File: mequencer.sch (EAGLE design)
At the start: 62 parts, among them IC1 NE555D, IC10 LF353D, IC11 NE555D, IC12 NE555D, IC2 4163D, IC3 74HC85D, IC4 4051D, IC5 4051D, IC6 74HCT04D, IC7 4051D, IC8 4051D, IC9 LF353D, U1 74LVC1G08SE-7

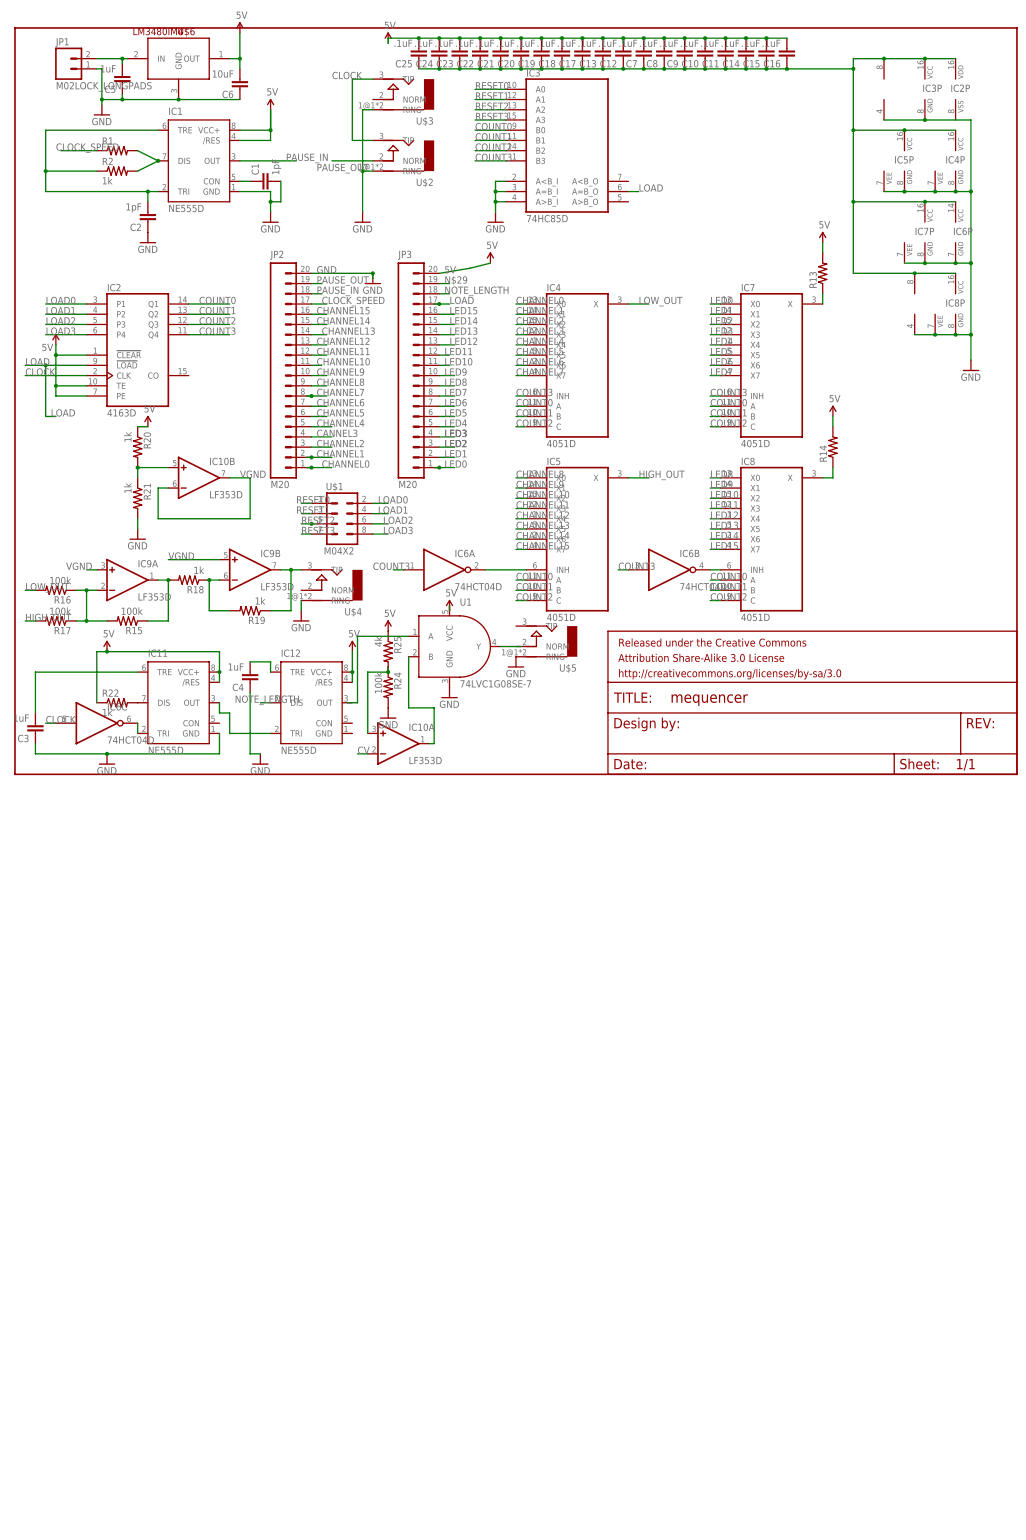
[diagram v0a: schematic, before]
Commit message: mini boards
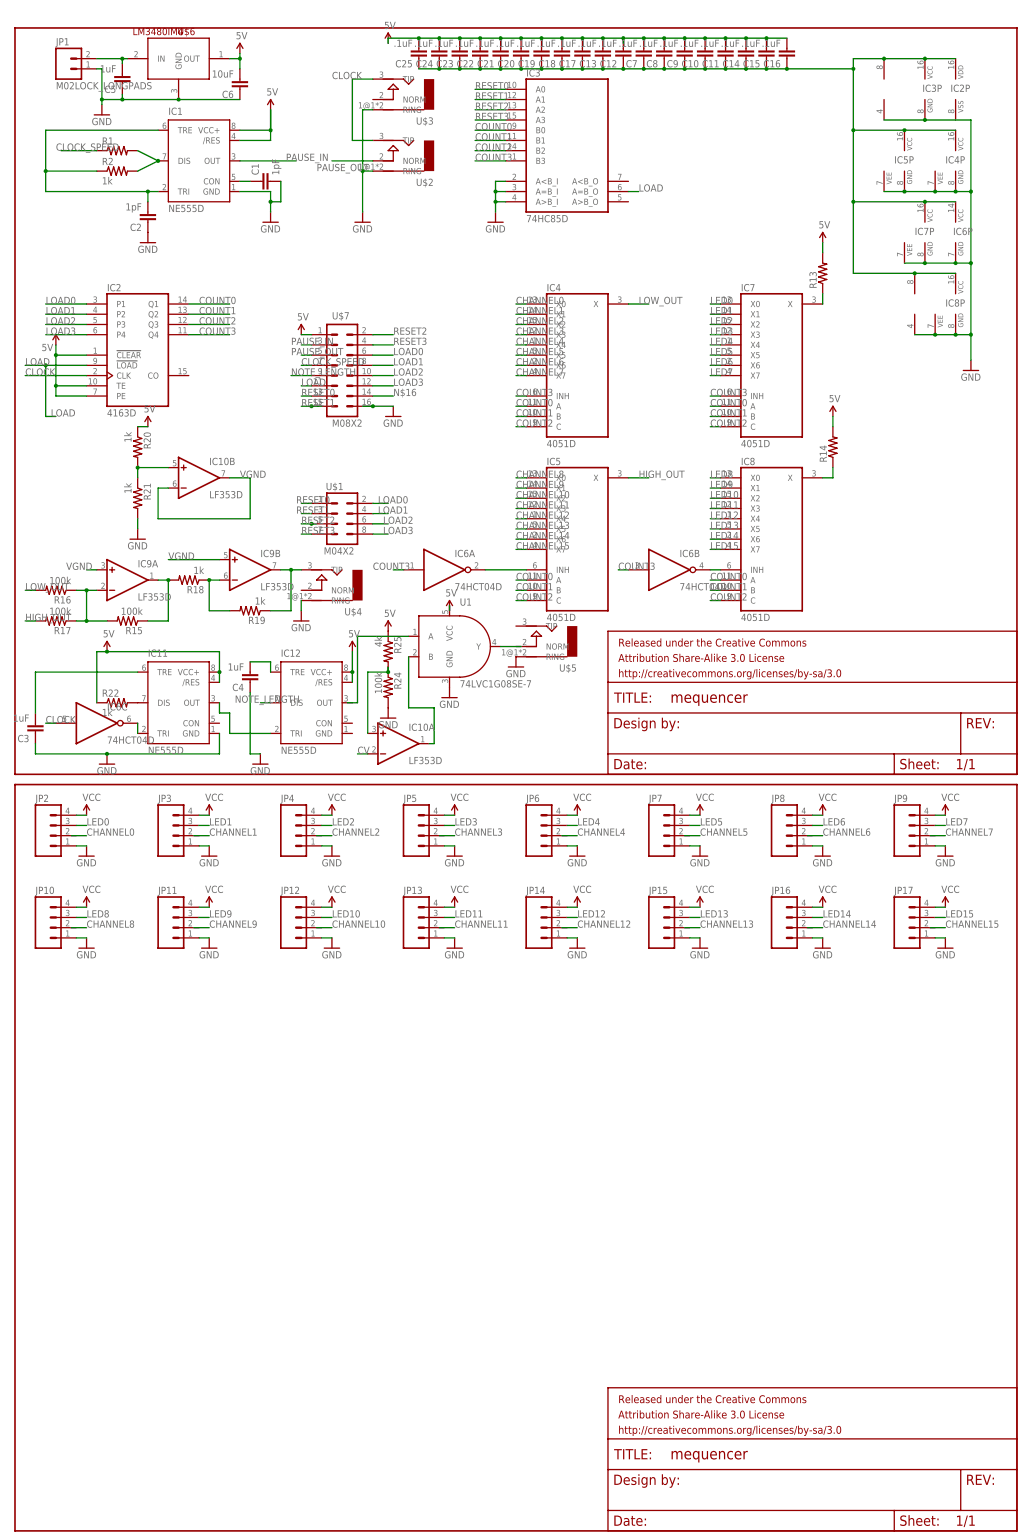
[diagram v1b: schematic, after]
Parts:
- added FRAME2: FRAME-LETTER, SparkFun-Aesthetics:FRAME-LETTER
- added JP10, JP11, JP12, JP13, JP14, JP15, JP16, JP17, JP4, JP5, JP6, JP7, JP8, JP9: (no value), SparkFun-Connectors:M04JST-PTH
- added U$7: M08X2, SparkFun-Connectors:M08X2
- JP2, JP3: value M20 -> (none); device SparkFun-Connectors:M20 -> SparkFun-Connectors:M04JST-PTH
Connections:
- removed net CANNEL3: JP2.4
- removed net N$29: JP3.19
- new net VCC: JP10.4, JP11.4, JP12.4, JP13.4, JP14.4, JP15.4, JP16.4, JP17.4, JP2.4, JP3.4, JP4.4, JP5.4, JP6.4, JP7.4, JP8.4, JP9.4
- net 5V: now also U$7.1; no longer JP3.20
- net CHANNEL0: no longer JP2.1
- net CHANNEL1: no longer JP2.2
- net CHANNEL10: no longer JP2.11
- net CHANNEL11: no longer JP2.12
- net CHANNEL12: no longer JP2.13
- net CHANNEL13: no longer JP2.14
- net CHANNEL14: no longer JP2.15
- net CHANNEL15: no longer JP2.16
- net CHANNEL2: no longer JP2.3
- net CHANNEL4: no longer JP2.5
- net CHANNEL5: no longer JP2.6
- net CHANNEL6: no longer JP2.7
- net CHANNEL7: no longer JP2.8
- net CHANNEL8: no longer JP2.9
- net CHANNEL9: no longer JP2.10
- net CLOCK_SPEED: now also U$7.7; no longer JP2.17
- net GND: now also JP10.1, JP11.1, JP12.1, JP13.1, JP14.1, JP15.1, JP16.1, JP17.1, JP2.1, JP3.1, JP4.1, JP5.1, JP6.1, JP7.1, JP8.1, JP9.1, U$7.16; no longer JP2.20
- net LED0: now also JP2.3; no longer JP3.1
- net LED1: now also JP3.3; no longer JP3.2
- net LED10: now also JP12.3; no longer JP3.11
- net LED11: now also JP13.3; no longer JP3.12
- net LED12: now also JP14.3; no longer JP3.13
- net LED13: now also JP15.3; no longer JP3.14
- net LED14: now also JP16.3; no longer JP3.15
- net LED15: now also JP17.3; no longer JP3.16
- net LED2: now also JP4.3; no longer JP3.3
- net LED3: now also JP5.3; no longer JP3.4
- net LED4: now also JP6.3; no longer JP3.5
- net LED5: now also JP7.3; no longer JP3.6
- net LED6: now also JP8.3; no longer JP3.7
- net LED7: now also JP9.3; no longer JP3.8
- net LED8: now also JP10.3; no longer JP3.9
- net LED9: now also JP11.3; no longer JP3.10
- net LOAD: now also U$7.11; no longer JP3.17
- net LOAD0: now also U$7.6
- net LOAD1: now also U$7.8
- net LOAD2: now also U$7.10
- net LOAD3: now also U$7.12
- net N$16: now also U$7.14
- net NOTE_LENGTH: now also U$7.9; no longer JP3.18
- net PAUSE_IN: now also U$7.3; no longer JP2.18
- net PAUSE_OUT: now also U$7.5; no longer JP2.19
- net RESET0: now also U$7.13
- net RESET1: now also U$7.15
- net RESET2: now also U$7.2
- net RESET3: now also U$7.4
